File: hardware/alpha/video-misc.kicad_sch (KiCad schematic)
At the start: 30 parts, among them P30 BANK2_AUX, U1 74LVCH16T245, U1 L78L05_SO8, U3 74LVC1T45, U3 L79L05_SO8, U6 TLE2082, U8 MCP47FEB22A0-E/ST

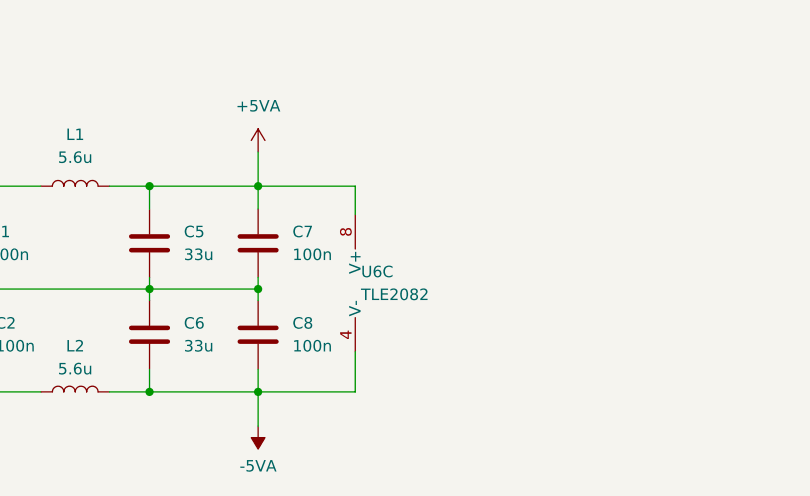
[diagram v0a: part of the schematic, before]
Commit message: WIP
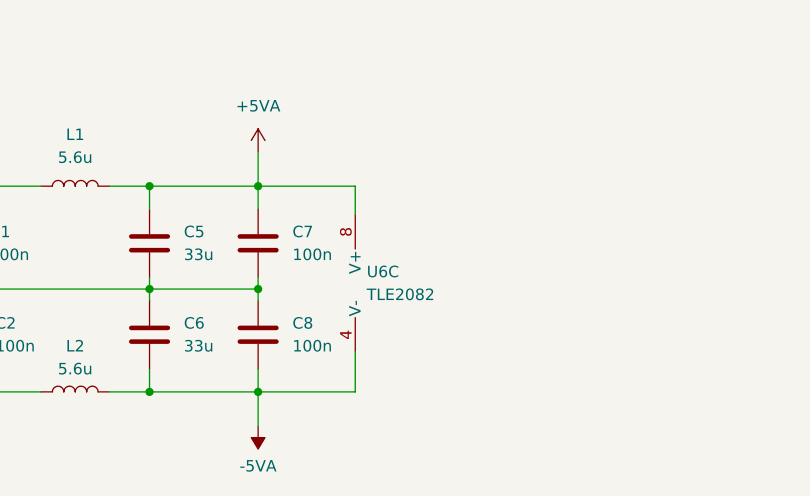
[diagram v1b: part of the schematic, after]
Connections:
- net +3.3VP renamed +3.3V_HACKRF
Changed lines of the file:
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@@
   (symbol (lib_id "Amplifier_Operational:AD8620") (at 147.32 154.305 0) (unit 3)
     (in_bom yes) (on_board yes) (dnp no) (fields_autoplaced)
-    (property "Reference" "U6" (at 145.415 153.035 0)
+    (property "Reference" "U6" (at 146.05 153.035 0)
       (effects (font (size 1.27 1.27)) (justify left))
     )
-    (property "Value" "TLE2082" (at 145.415 155.575 0)
+    (property "Value" "TLE2082" (at 146.05 155.575 0)
       (effects (font (size 1.27 1.27)) (justify left))
     )
@@
         )
         (path "/487245ca-0c1f-4f9d-bc99-20c8f558090f/e1e307fe-d49b-45b6-b177-774a7a482979"
-          (reference "U16") (unit 3)
+          (reference "U6") (unit 3)
         )
       )

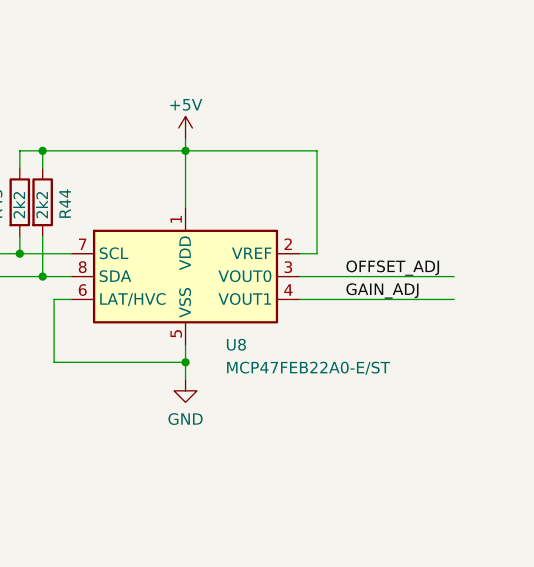
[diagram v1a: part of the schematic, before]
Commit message: WIP
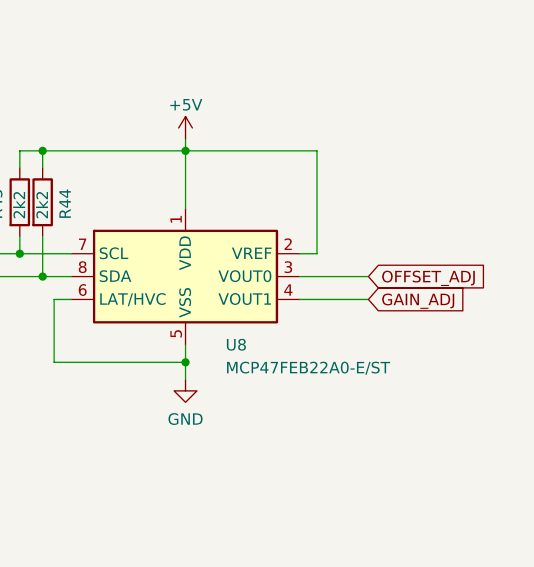
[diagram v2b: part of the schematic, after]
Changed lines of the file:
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@@
     (stroke (width 0) (type default))
   )
-  (wire (pts (xy 249.555 141.605) (xy 266.7 141.605))
+  (wire (pts (xy 249.555 141.605) (xy 257.175 141.605))
     (stroke (width 0) (type default))
   )
@@
     (stroke (width 0) (type default))
   )
-  (wire (pts (xy 249.555 144.145) (xy 266.7 144.145))
+  (wire (pts (xy 249.555 144.145) (xy 257.175 144.145))
     (stroke (width 0) (type default))
   )
@@
     (effects (font (size 1.27 1.27)) (justify left bottom))
   )
-  (label "GAIN_ADJ" (at 254.635 144.145 0) (fields_autoplaced)
-    (effects (font (size 1.27 1.27)) (justify left bottom))
-  )
   (label "LAD4" (at 89.535 64.77 0) (fields_autoplaced)
     (effects (font (size 1.27 1.27)) (justify left bottom))
@@
   )
   (label "LAD11" (at 62.23 76.2 0) (fields_autoplaced)
-    (effects (font (size 1.27 1.27)) (justify left bottom))
-  )
-  (label "OFFSET_ADJ" (at 254.635 141.605 0) (fields_autoplaced)
     (effects (font (size 1.27 1.27)) (justify left bottom))
   )
@@
     )
   )
+  (global_label "GAIN_ADJ" (shape input) (at 257.175 144.145 0) (fields_autoplaced)
+    (effects (font (size 1.27 1.27)) (justify left))
+    (property "Intersheetrefs" "${INTERSHEET_REFS}" (at 268.7479 144.145 0)
+      (effects (font (size 1.27 1.27)) (justify left) hide)
+    )
+  )
+  (global_label "OFFSET_ADJ" (shape input) (at 257.175 141.605 0) (fields_autoplaced)
+    (effects (font (size 1.27 1.27)) (justify left))
+    (property "Intersheetrefs" "${INTERSHEET_REFS}" (at 271.2878 141.605 0)
+      (effects (font (size 1.27 1.27)) (justify left) hide)
+    )
+  )

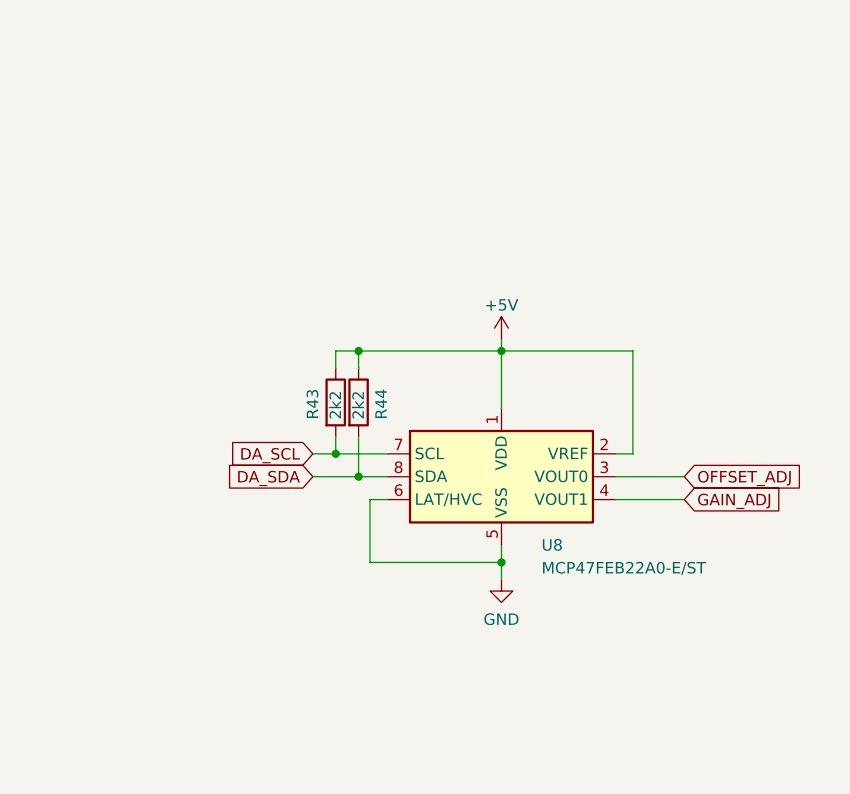
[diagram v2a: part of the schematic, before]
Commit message: WIP
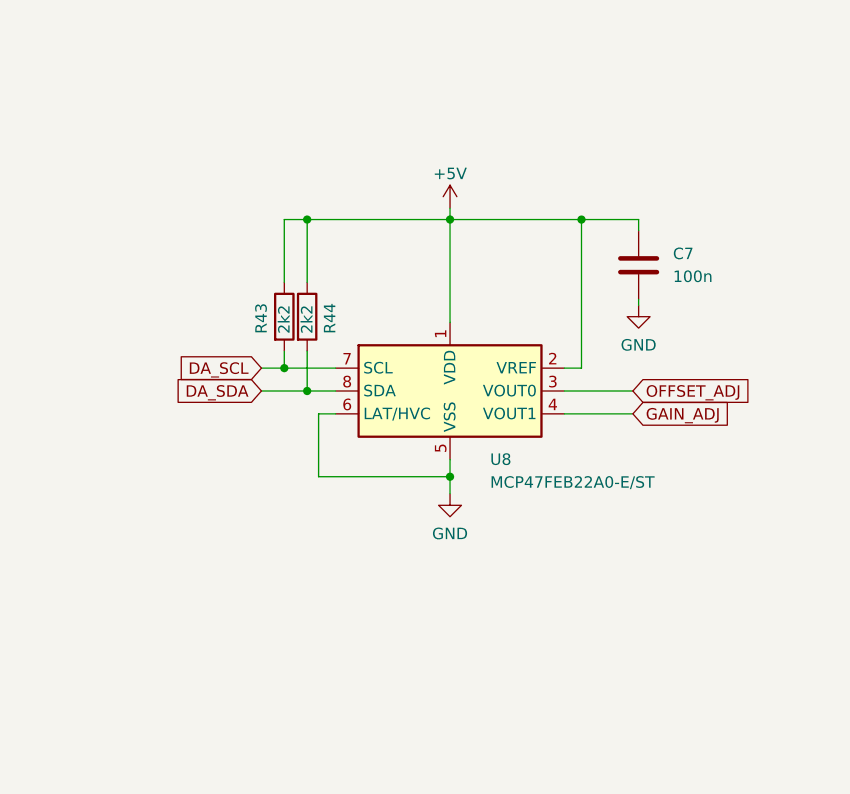
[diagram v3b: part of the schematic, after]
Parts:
- added C7: 100n, Capacitor_SMD:C_0603_1608Metric, symbol Device:C
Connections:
- net +5V: now also C7.1
- net GND: now also C7.2
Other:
- moved on the sheet: R43, R44, U8

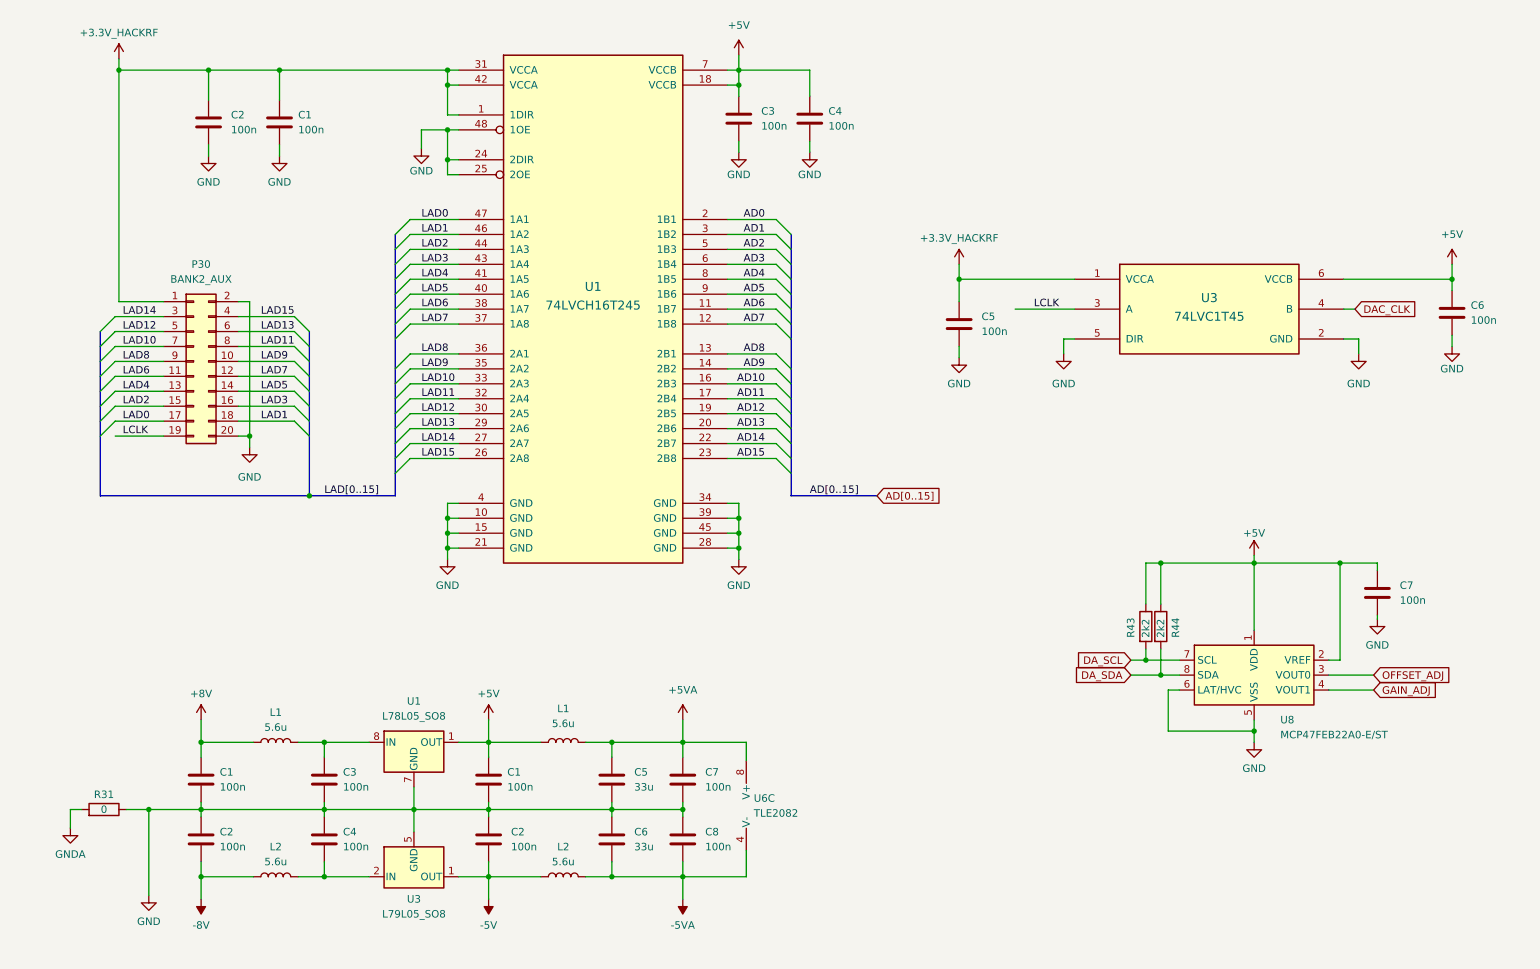
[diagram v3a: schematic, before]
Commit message: WIP
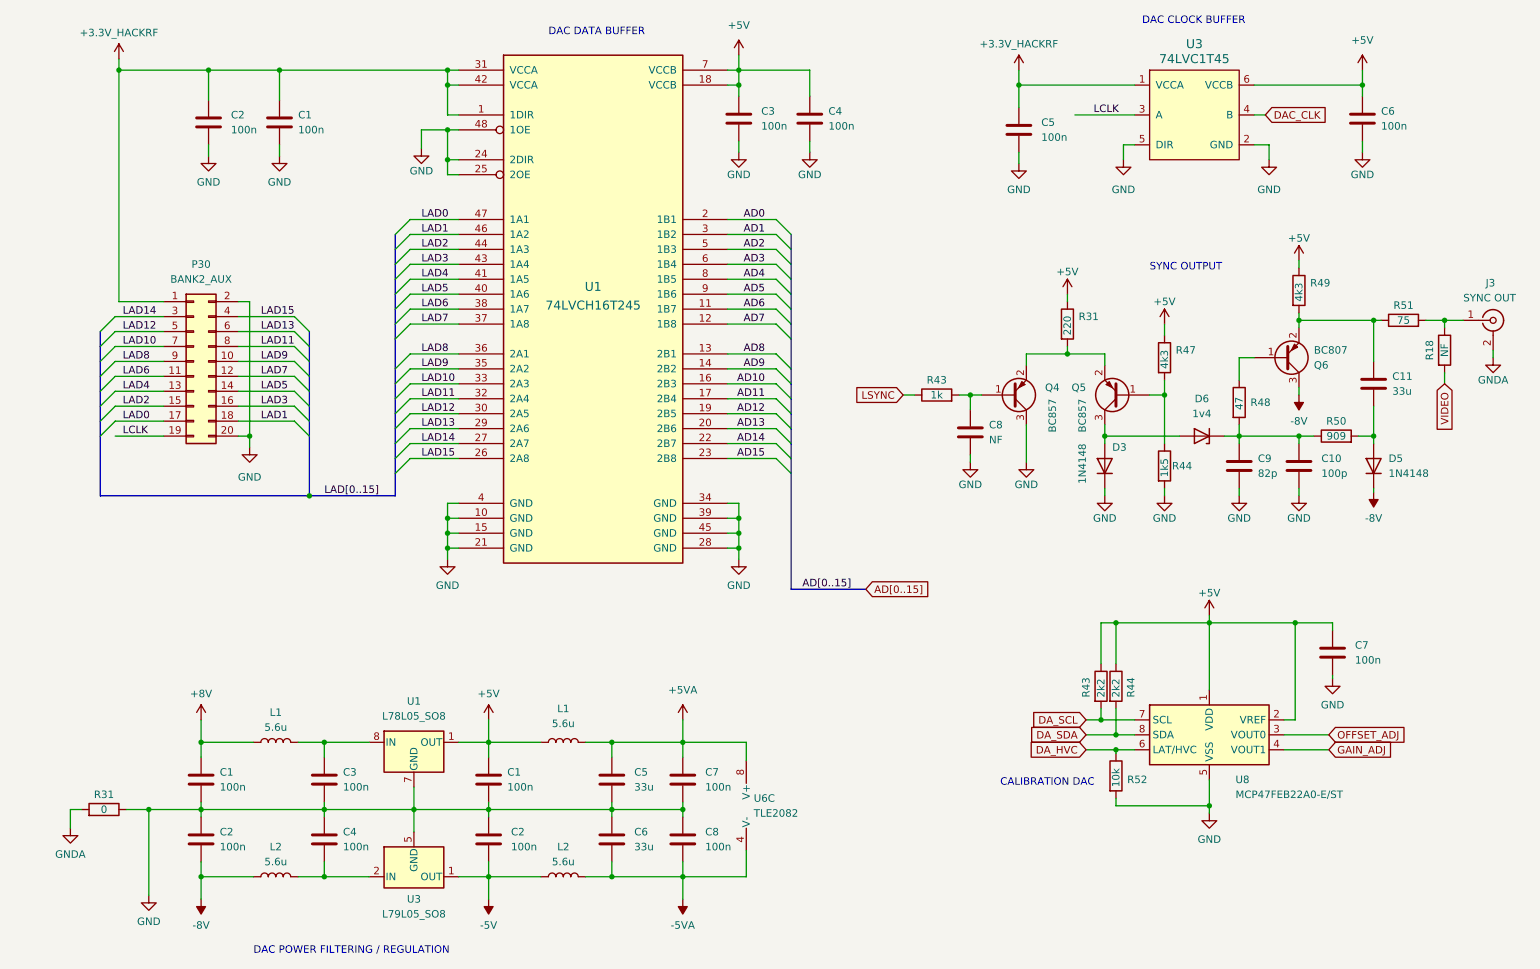
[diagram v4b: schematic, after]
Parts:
- added C10: 100p, symbol Device:C
- added C11: 33u, symbol Device:C
- added C8: NF, symbol Device:C
- added C9: 82p, symbol Device:C
- added D3, D5: 1N4148, Diode_SMD:D_SOD-123, symbol Device:D
- added D6: 1v4, Package_TO_SOT_SMD:SOT-23, symbol Diode:BZX84Cxx
- added J3: SYNC OUT, MOLEX_73101:731010120, symbol Connector:Conn_Coaxial
- added Q4, Q5: BC857, Package_TO_SOT_SMD:SOT-23, symbol Transistor_BJT:BC857
- added Q6: BC807, Package_TO_SOT_SMD:SOT-23, symbol Transistor_BJT:BC807
- added R18: NF, Resistor_SMD:R_0603_1608Metric, symbol Device:R
- added R31: 220, Resistor_SMD:R_0603_1608Metric, symbol Device:R
- added R43: 1k, Resistor_SMD:R_0603_1608Metric, symbol Device:R
- added R44: 1k5, Resistor_SMD:R_0603_1608Metric, symbol Device:R
- added R47, R49: 4k3, Resistor_SMD:R_0603_1608Metric, symbol Device:R
- added R48: 47, Resistor_SMD:R_0603_1608Metric, symbol Device:R
- added R50: 909, Resistor_SMD:R_0603_1608Metric, symbol Device:R
- added R51: 75, Resistor_SMD:R_0603_1608Metric, symbol Device:R
- added R52: 10k, Resistor_SMD:R_0603_1608Metric, symbol Device:R
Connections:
- net +5V: now also R31.1, R47.1, R49.1
- net -8V: now also D5.1 (K), Q6.3 (C)
- net GND: now also C10.2, C8.2, C9.2, D3.1 (K), Q4.3 (C), R44.2, R52.2; no longer U8.6 (LAT/HVC)
- net GNDA: now also J3.2 (Ext)
- new net: C11.2, D5.2 (A), R50.2
- new net: C8.1, Q4.1 (B), R43.2
- new net: Q6.1 (B), R48.1
- new net: C10.1, C9.1, D6.3 (K), R48.2, R50.1
- new net: C11.1, Q6.2 (E), R49.2, R51.1
- new net: J3.1 (In), R18.1, R51.2
- new net: D3.2 (A), D6.1 (A), Q5.3 (C)
- new net: Q4.2 (E), Q5.2 (E), R31.2
- new net: Q5.1 (B), R44.1, R47.2
- new net DA_HVC: R52.1, U8.6 (LAT/HVC)
- new net LSYNC: R43.1
- new net VIDEO: R18.2
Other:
- note added: "CALIBRATION DAC"
- note added: "DAC CLOCK BUFFER"
- note added: "DAC DATA BUFFER"
- note added: "DAC POWER FILTERING / REGULATION"
- note added: "SYNC OUTPUT"
- moved on the sheet: C5, C6, C7, R43, R44, U3, U8

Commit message: WIP
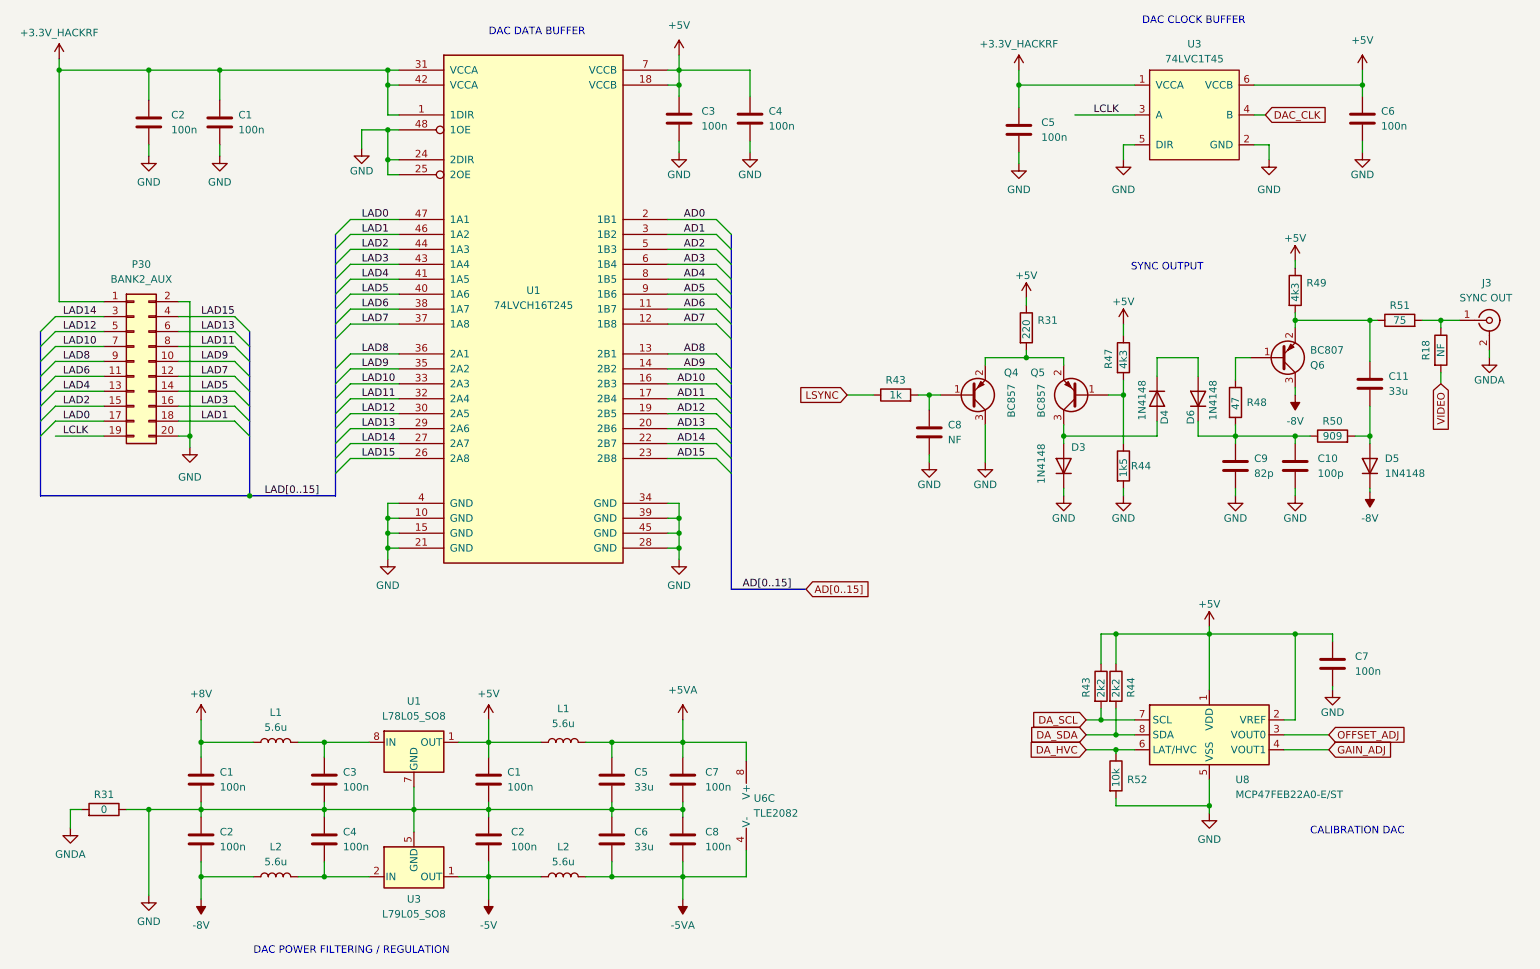
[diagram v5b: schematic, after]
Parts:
- removed D6: 1v4, Package_TO_SOT_SMD:SOT-23, symbol Diode:BZX84Cxx
- added D4, D6: 1N4148, Diode_SMD:D_SOD-123, symbol Device:D
- C10, C8, C9: footprint (none) -> Capacitor_SMD:C_0603_1608Metric
- C11: footprint (none) -> Capacitor_SMD:C_1210_3225Metric
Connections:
- net at C10.1, C9.1, R48.2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: now also D6.1 (K)
- net at D3.2 (A), Q5.3 (C): now also D4.2 (A)
- new net: D4.1 (K), D6.2 (A)
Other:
- moved on the sheet: C1, C10, C11, C2, C3, C4, C7, C8, C9, D3, D5, J3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
